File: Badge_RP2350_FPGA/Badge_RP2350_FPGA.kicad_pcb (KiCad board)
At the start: 2 copper layers, 100 x 150 mm, 100 parts, among them J1 USB_C_Receptacle_USB2.0_16P, J2 Conn_01x03_Pin, J3 Conn_01x15_Pin, J4 Conn_01x15_Pin, SW1 SW_Push, SW12 On/Off, SW2 SW_Push, U1 RP2350_60QFN, U2 GW1N-LV9QN88C6_I5_, U3 ME6211C12, U4 TMI7003C, U6 W25Q32JVSS, U7 W25Q32JVSS, Y1 ABM8-272-T3

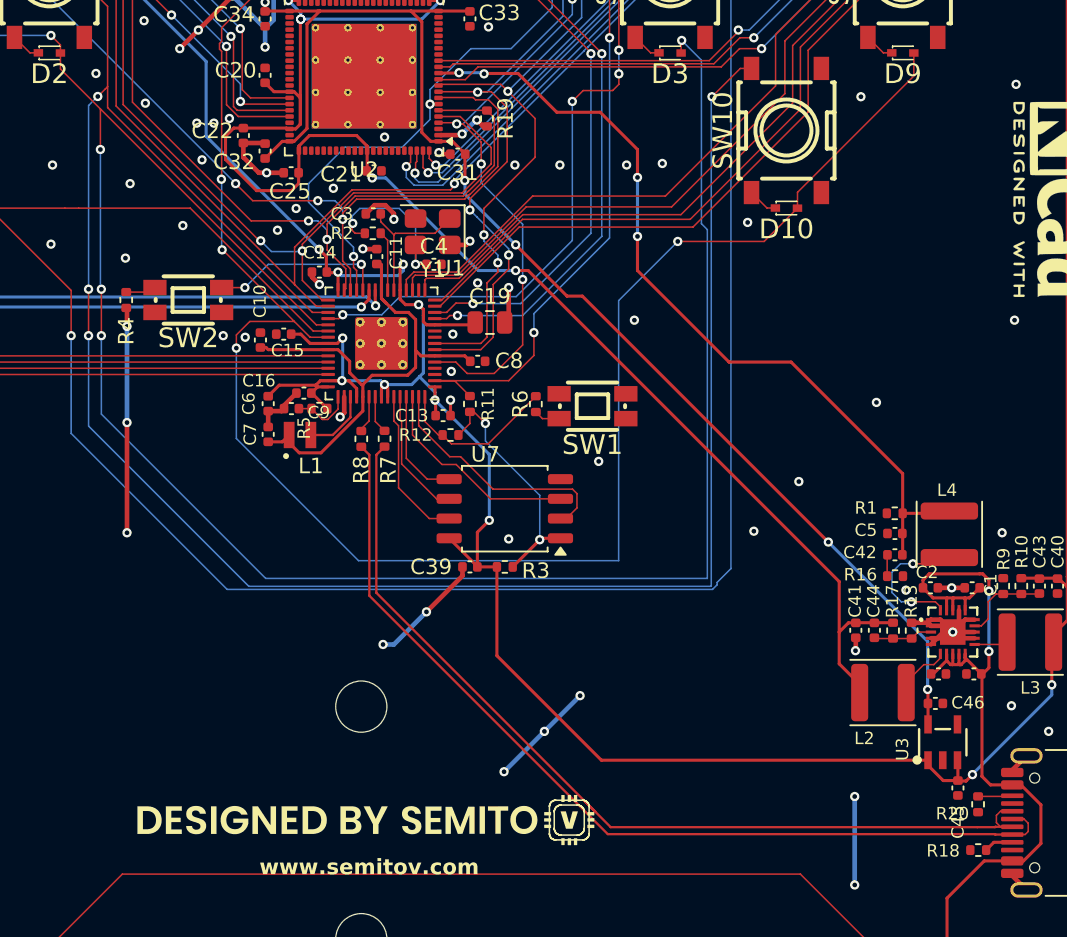
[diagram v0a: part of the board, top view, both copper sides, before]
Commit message: fix a bunch of stuff
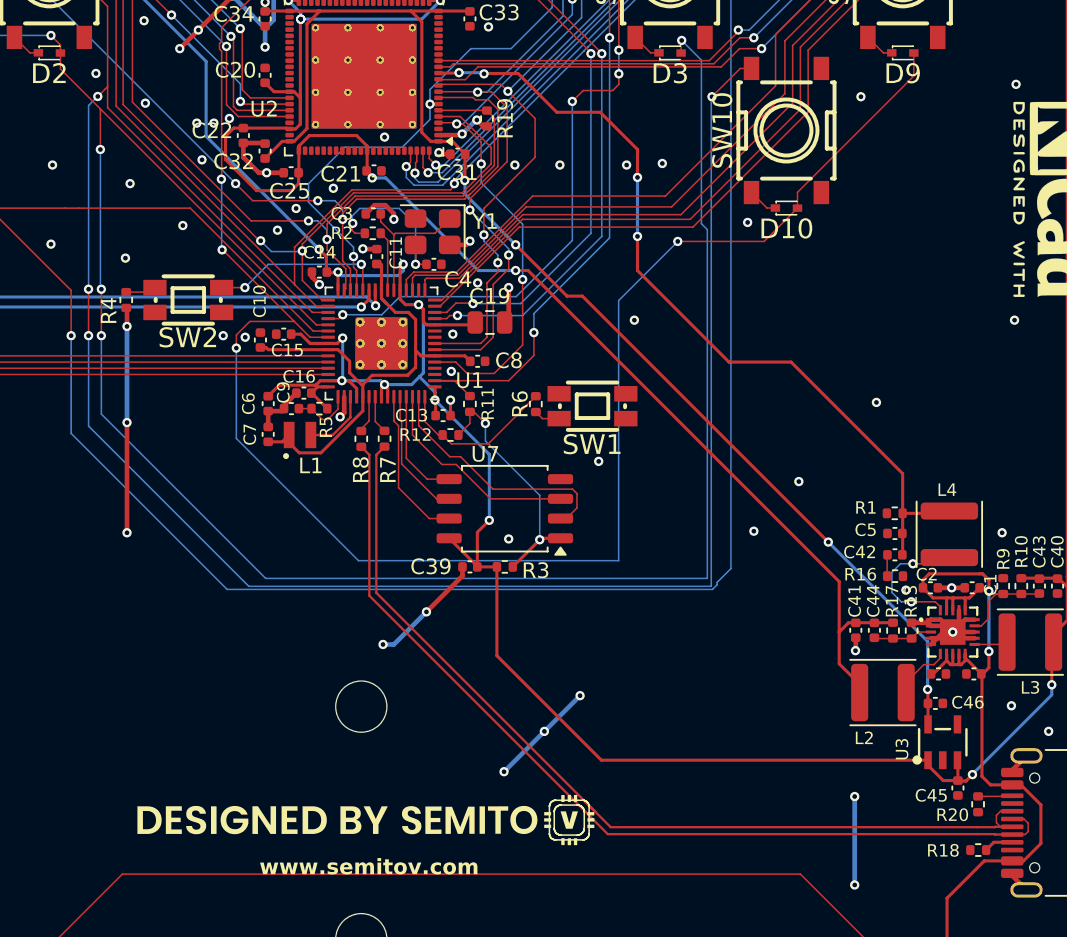
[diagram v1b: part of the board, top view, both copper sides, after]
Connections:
- net /GW1NR 9K FPGA/MCLK renamed /GW1N 9K FPGA/MCLK
- net /GW1NR 9K FPGA/MCS_N renamed /GW1N 9K FPGA/MCS_N
- net /GW1NR 9K FPGA/MISO_SD1 renamed /GW1N 9K FPGA/MISO_SD1
- net /GW1NR 9K FPGA/MOSI_SD0 renamed /GW1N 9K FPGA/MOSI_SD0
